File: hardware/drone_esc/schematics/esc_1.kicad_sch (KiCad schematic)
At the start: 32 parts, among them Q1 BSC016N04LS, Q2 BSC016N04LS, Q3 BSC016N04LS, Q4 BSC016N04LS, Q5 BSC016N04LS, Q6 BSC016N04LS, U4 FD6288Q

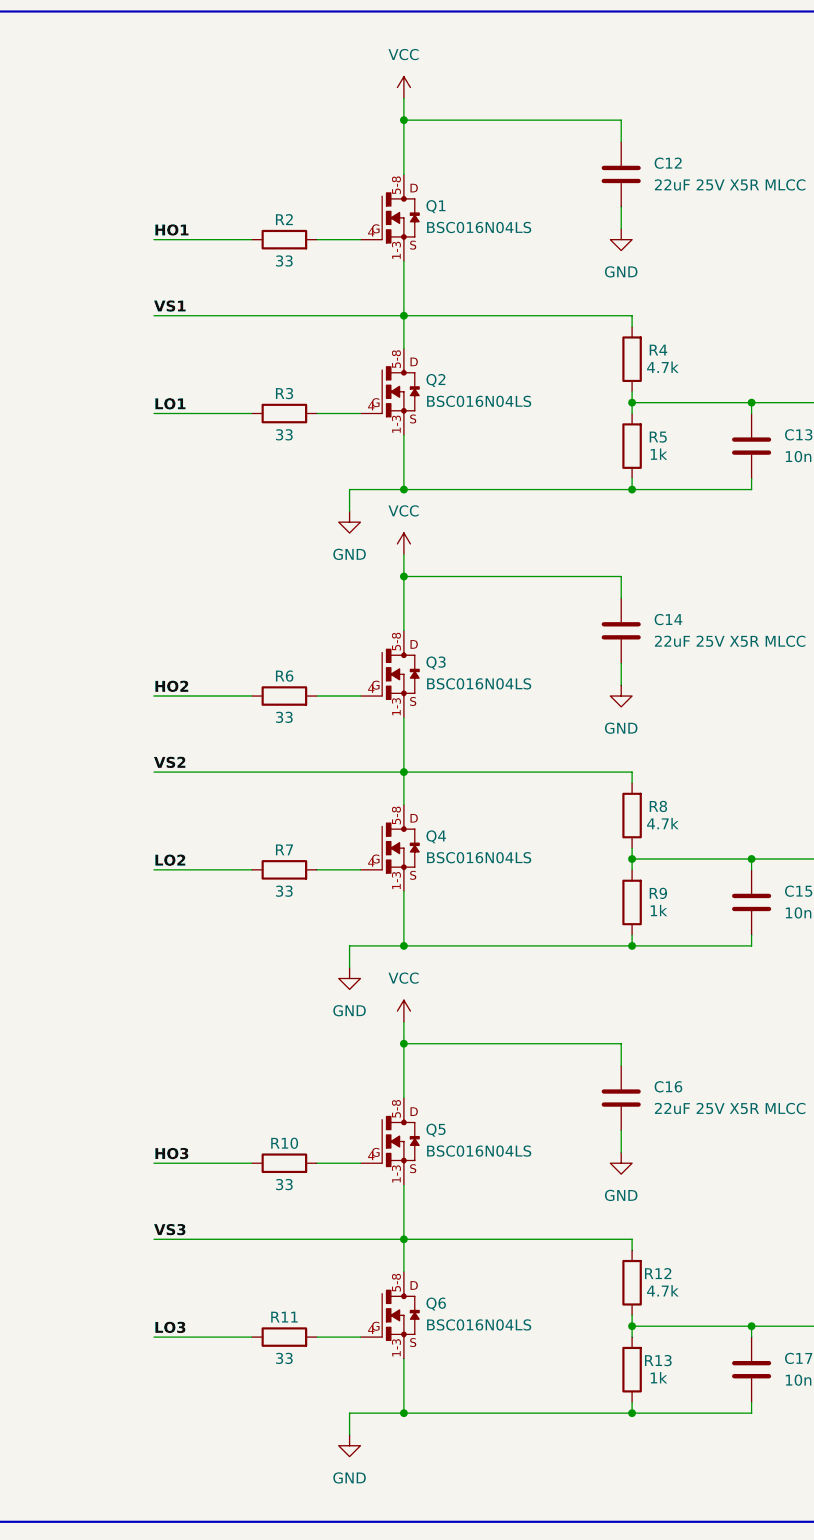
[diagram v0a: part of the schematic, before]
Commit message: replaced some of the schematics
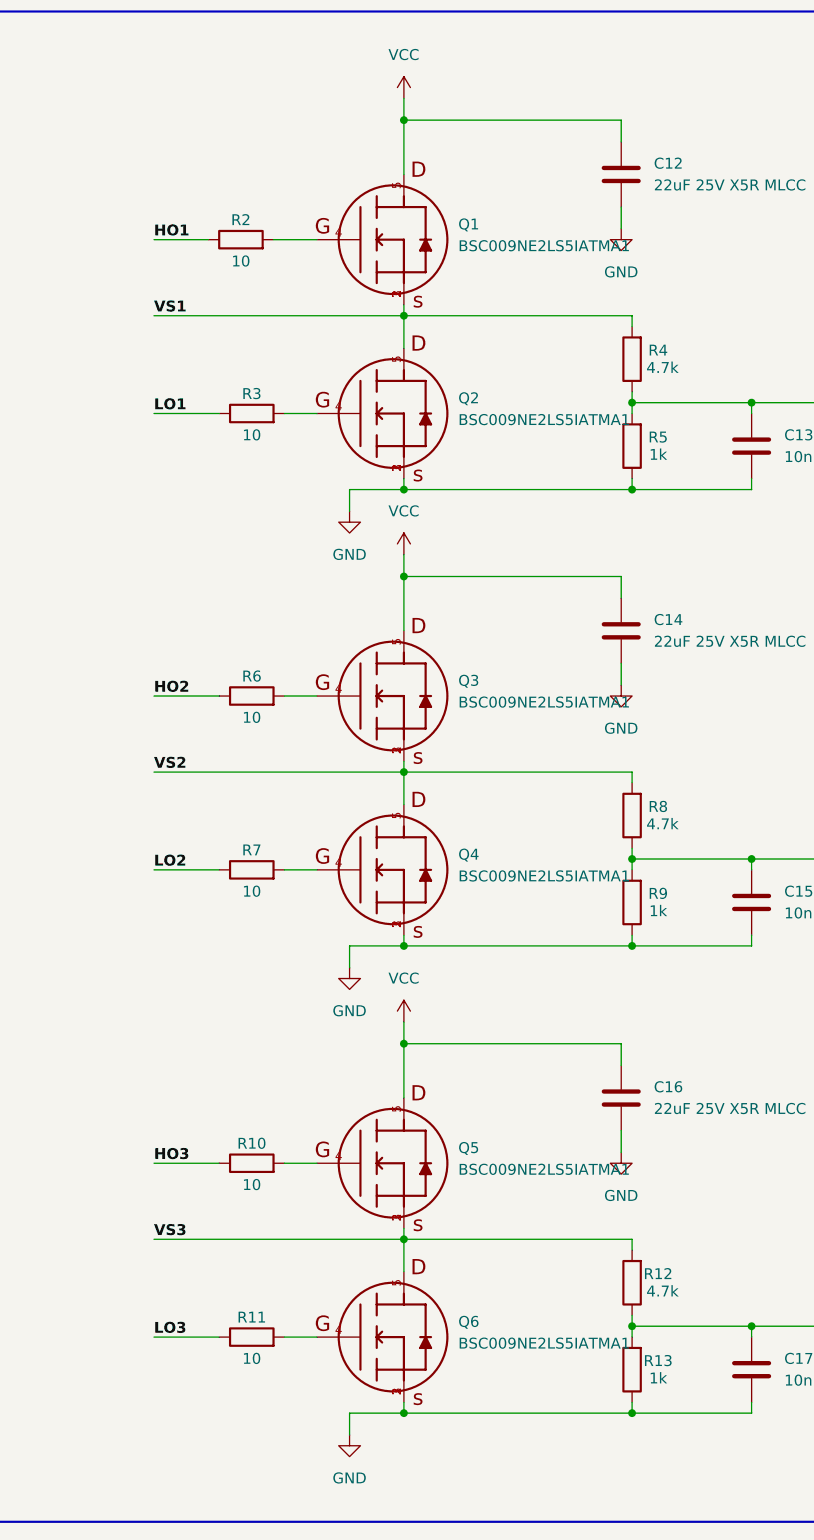
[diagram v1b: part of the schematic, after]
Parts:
- removed Q1, Q2, Q3, Q4, Q5, Q6: BSC016N04LS, Drone_components:BSC016N04LS, symbol Drone_components:BSC016N04LS
- added Q1, Q2, Q3, Q4, Q5, Q6: BSC009NE2LS5IATMA1, Drone_components:BSC093N04LSGATMA1, symbol Drone_components:BSC009NE2LS5IATMA1
- C12, C14, C16: footprint Capacitor_SMD:C_1210_3225Metric -> Capacitor_SMD:C_0805_2012Metric; JLCPCB part C12891 -> C45783
- R10, R11, R2, R3, R6, R7: value 33 -> 10
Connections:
- net GND: now also Q2.1, Q2.2, Q2.3, Q4.1, Q4.2, Q4.3, Q6.1, Q6.2, Q6.3
- net VCC: now also Q1.5, Q3.5, Q5.5
- net VS1: now also Q1.1, Q1.2, Q1.3, Q2.5
- net VS2: now also Q3.1, Q3.2, Q3.3, Q4.5
- net VS3: now also Q5.1, Q5.2, Q5.3, Q6.5
- net at R11.2: now also Q6.4
- net at R2.2: now also Q1.4
- net at R10.2: now also Q5.4
- net at R3.2: now also Q2.4
- net at R6.2: now also Q3.4
- net at R7.2: now also Q4.4
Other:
- moved on the sheet: R10, R11, R2, R3, R6, R7
